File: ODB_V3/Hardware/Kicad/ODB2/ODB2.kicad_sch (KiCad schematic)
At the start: 74 parts, among them U1 STM32F412ZGTx, Y1 ABM8G-25.000MHZ-18-D2Y-T

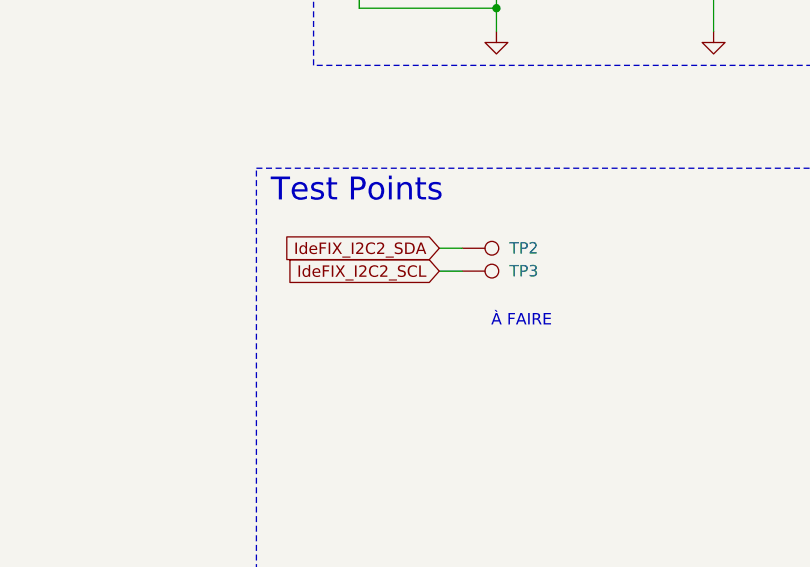
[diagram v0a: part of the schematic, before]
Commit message: wip: fix chainfreiner zone
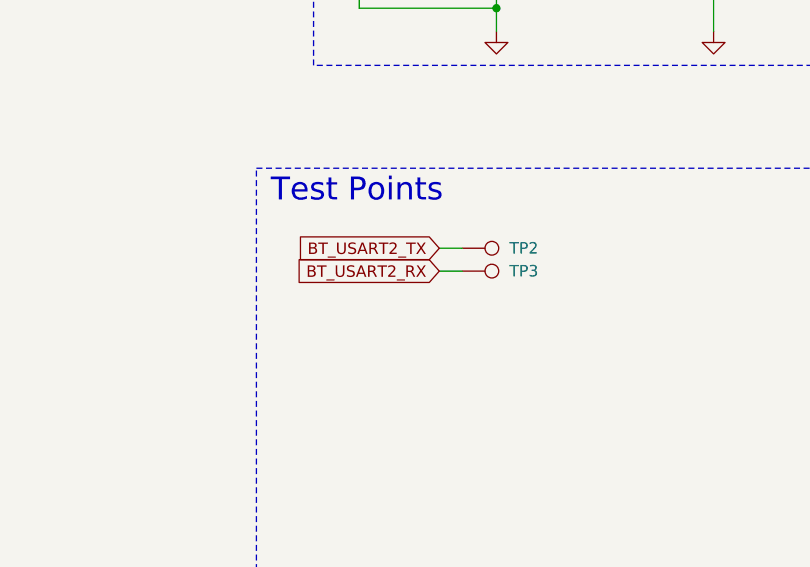
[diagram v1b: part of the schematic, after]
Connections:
- net BT_USART2_RX: now also TP3.1
- net BT_USART2_TX: now also TP2.1
- net IdeFIX_I2C2_SCL: no longer TP3.1
- net IdeFIX_I2C2_SDA: no longer TP2.1
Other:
- note removed: "À FAIRE"
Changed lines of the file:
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@@
 		)
 	)
-	(text "À FAIRE"
-		(exclude_from_sim no)
-		(at 368.554 222.758 0)
-		(effects
-			(font
-				(size 1.27 1.27)
-			)
-		)
-	)
 	(junction
 		(at 187.96 44.45)
@@
 		)
 	)
-	(global_label "IdeFIX_I2C2_SCL"
+	(global_label "BT_USART2_RX"
 		(shape input)
 		(at 359.41 217.17 180)
@@
 		)
 		(property "Intersheetrefs" "${INTERSHEET_REFS}"
-			(at 340.9429 217.17 0)
+			(at 342.6968 217.17 0)
 			(effects
 				(font
@@
 		)
 	)
-	(global_label "IdeFIX_I2C2_SDA"
+	(global_label "BT_USART2_TX"
 		(shape input)
 		(at 359.41 214.63 180)
@@
 		)
 		(property "Intersheetrefs" "${INTERSHEET_REFS}"
-			(at 340.8824 214.63 0)
+			(at 342.9992 214.63 0)
 			(effects
 				(font
